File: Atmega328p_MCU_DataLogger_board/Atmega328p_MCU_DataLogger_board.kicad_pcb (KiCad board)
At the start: 2 copper layers, 68.8 x 38.5 mm, 27 parts, among them J1 Conn_01x04_Pin, J2 Conn_01x04_Pin, J3 Conn_01x09_Pin, J4 Conn_02x03_Odd_Even, U1 24LC1025, U2 24LC1025, U3 ATMEGA328P-AU, U4 ds1337s+, Y1 Crystal, Y2 32.768 kHz

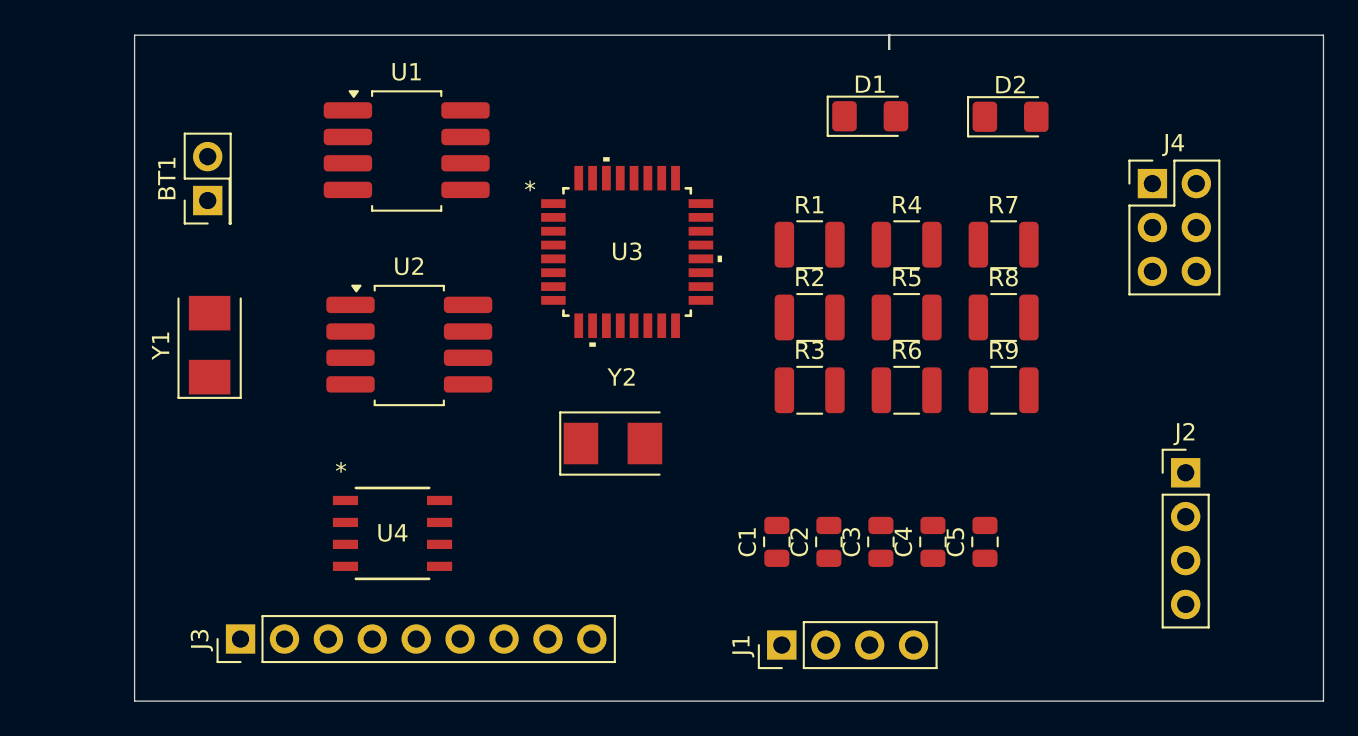
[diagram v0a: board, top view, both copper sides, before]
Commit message: Data Logger
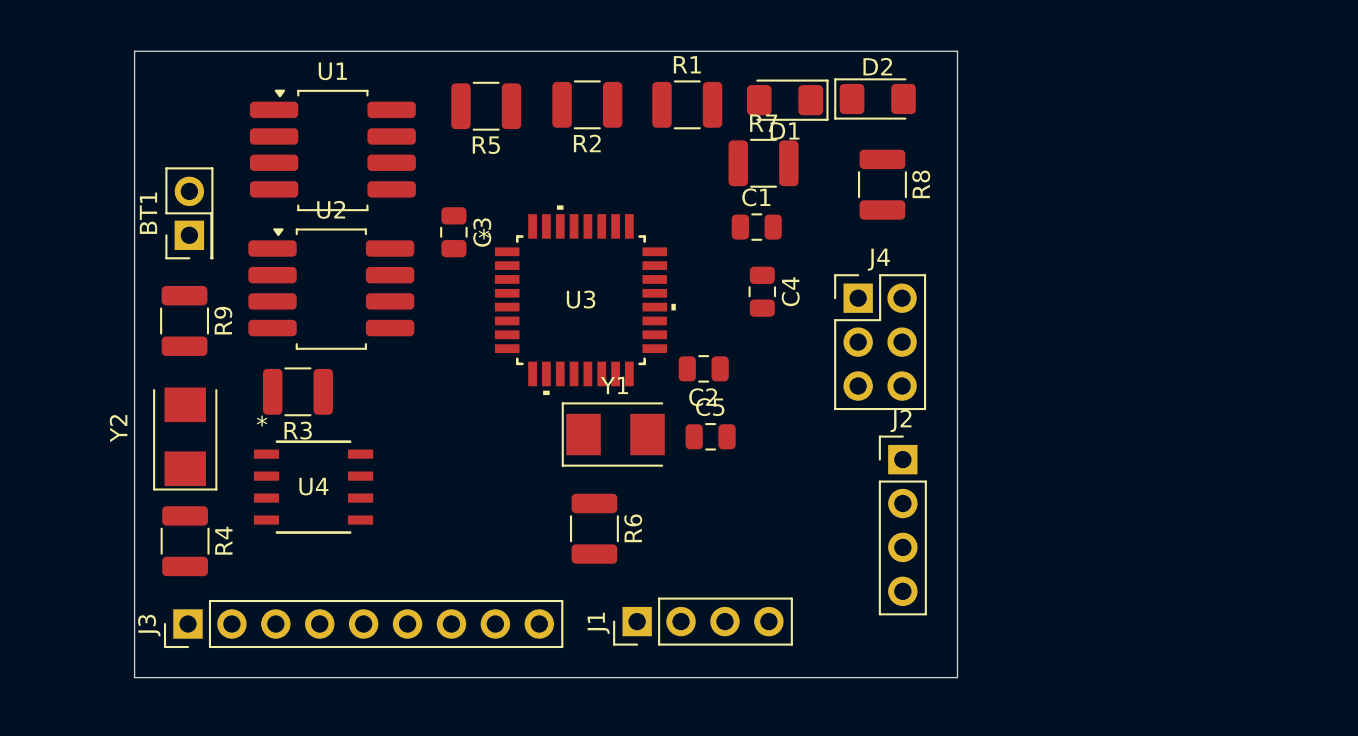
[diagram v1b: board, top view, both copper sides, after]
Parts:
- moved R9 47.5 mm to (48.6, 79.7), turned to -90 degrees
- moved R4 45.1 mm to (48.6, 92.5), turned to -90 degrees
- moved C3 30.5 mm to (64.1, 74.6), turned to -90 degrees
- moved R3 29.6 mm to (55.1, 83.8), turned to 180 degrees
- moved R5 27.2 mm to (66.0, 67.3), turned to 180 degrees
- moved Y2 24.7 mm to (48.6, 86.4), turned to 90 degrees
- moved Y1 24.0 mm to (73.5, 86.3), turned to 0 degrees
- moved R6 19.8 mm to (72.3, 91.8), turned to -90 degrees
- moved J4 18.3 mm to (87.5, 78.4)
- moved C1 18.2 mm to (81.7, 74.3), turned to 0 degrees
- moved R2 17.8 mm to (71.9, 67.2), turned to 180 degrees
- moved C4 17.5 mm to (82.0, 78.0), turned to -90 degrees
- moved C5 17.0 mm to (79.0, 86.4), turned to 0 degrees
- moved J2 16.4 mm to (90.1, 87.8)
- moved R7 14.7 mm to (82.0, 70.6)
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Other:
- board size 68.8 x 38.5 mm -> 47.6 x 36.2 mm

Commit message: Data Logger
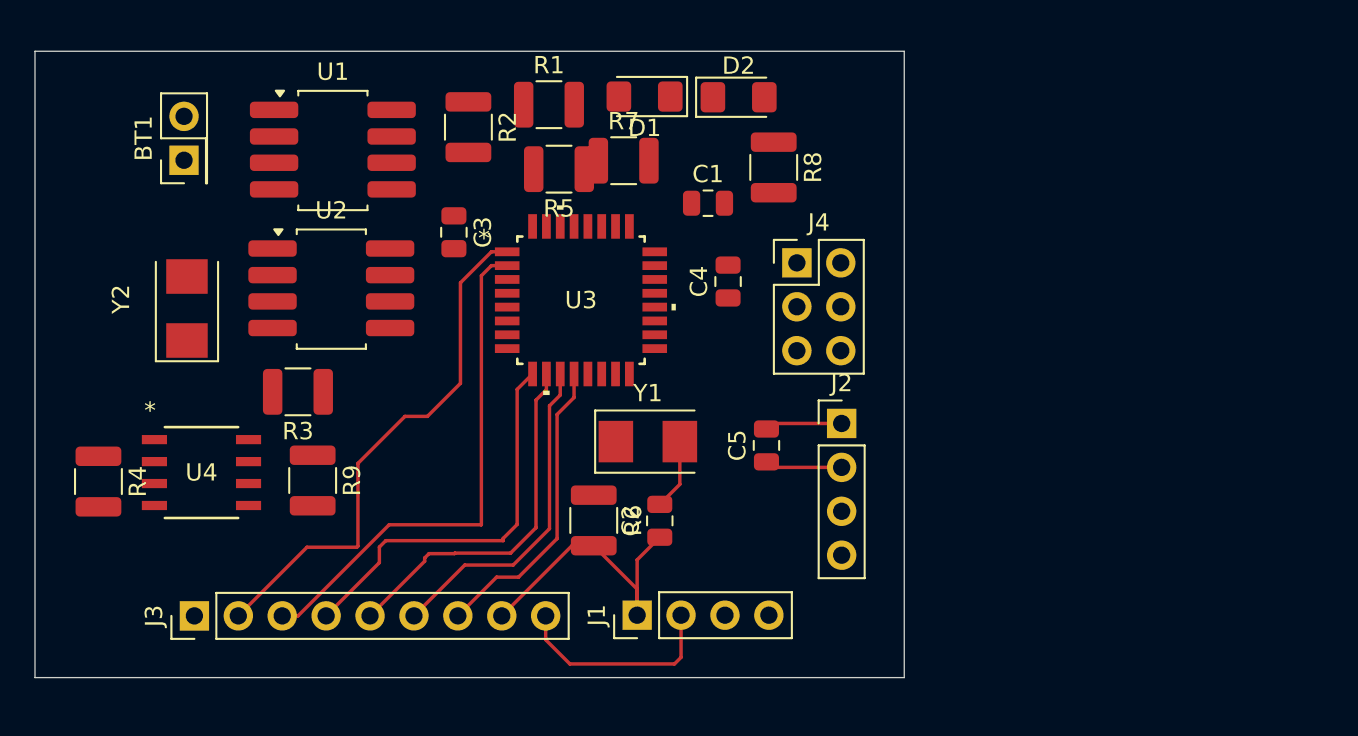
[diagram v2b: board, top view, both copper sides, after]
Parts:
- moved R9 11.8 mm to (56.0, 89.0)
- moved C2 9.15 mm to (76.0, 91.3), turned to 90 degrees
- moved D1 8.12 mm to (75.2, 66.8)
- moved R7 8.09 mm to (74.0, 70.5)
- moved D2 8.05 mm to (80.6, 66.8)
- moved R1 8.00 mm to (69.6, 67.2)
- moved Y2 7.42 mm to (48.7, 79.0)
- moved R2 7.00 mm to (65.0, 68.5), turned to -90 degrees
- moved U4 6.53 mm to (49.5, 88.5)
- moved R8 6.37 mm to (82.6, 70.9)
- moved R4 6.08 mm to (43.6, 89.0)
- moved R5 5.57 mm to (70.2, 71.0)
- moved BT1 4.35 mm to (48.5, 70.4)
- moved J2 4.11 mm to (86.6, 85.7)
- moved J4 4.09 mm to (84.0, 76.4)
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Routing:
- net D3: track 0.00 -> 30.5 mm
- net D4: track 0.00 -> 29.8 mm
- net D5: track 0.00 -> 22.9 mm
- net GND: track 0.00 -> 21.6 mm
- net D6: track 0.00 -> 21.0 mm
- net D7: track 0.00 -> 19.1 mm
- net D8: track 0.00 -> 17.5 mm
- net VCC: track 0.00 -> 16.9 mm
- net Net-(U3-PB6(PCINT6/XTAL1/TOSC1)): track 0.00 -> 4.11 mm
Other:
- board size 47.6 x 36.2 mm -> 50.3 x 36.2 mm
